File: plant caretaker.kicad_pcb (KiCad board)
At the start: 2 copper layers, 56 parts, among them J3 Water_Pump, J4 Kitronik, J5 694106402002, Q1 FDMS86255, U1 UDA1380HN_N2, U2 TMP175AIDR, U4 LM2596S-5, U5 PAM8403D, U6 ESP32_C3_ZERO

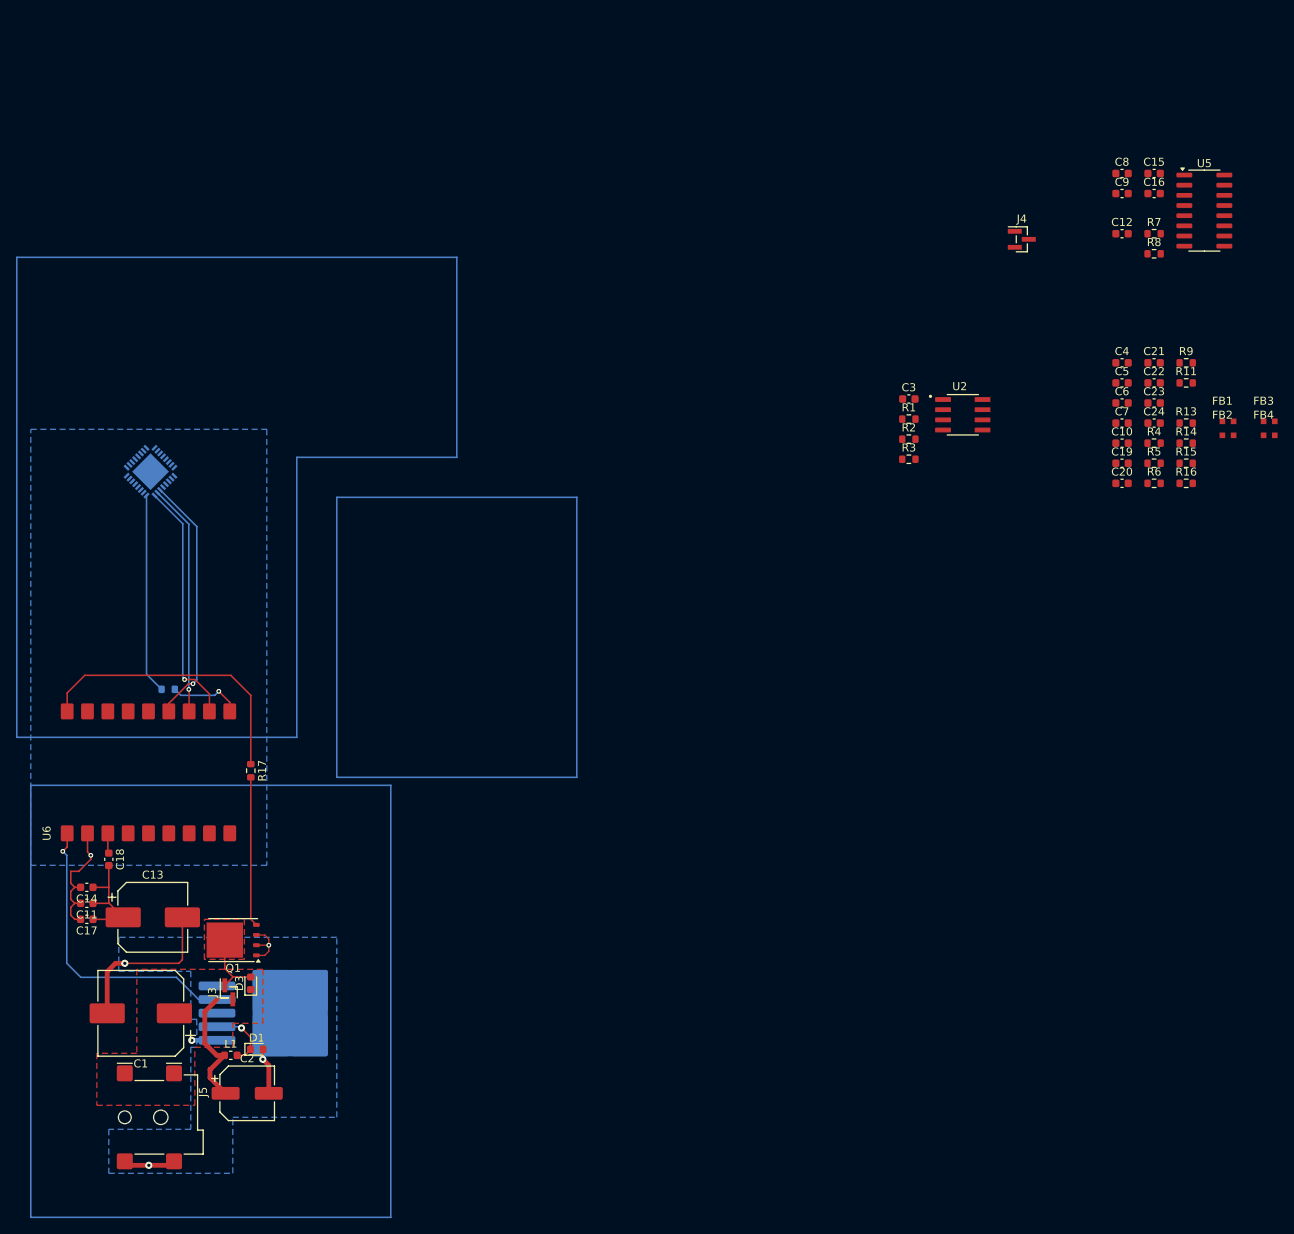
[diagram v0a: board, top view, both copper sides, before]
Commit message: Added more connections
Updated footprints for pin heads and speakers
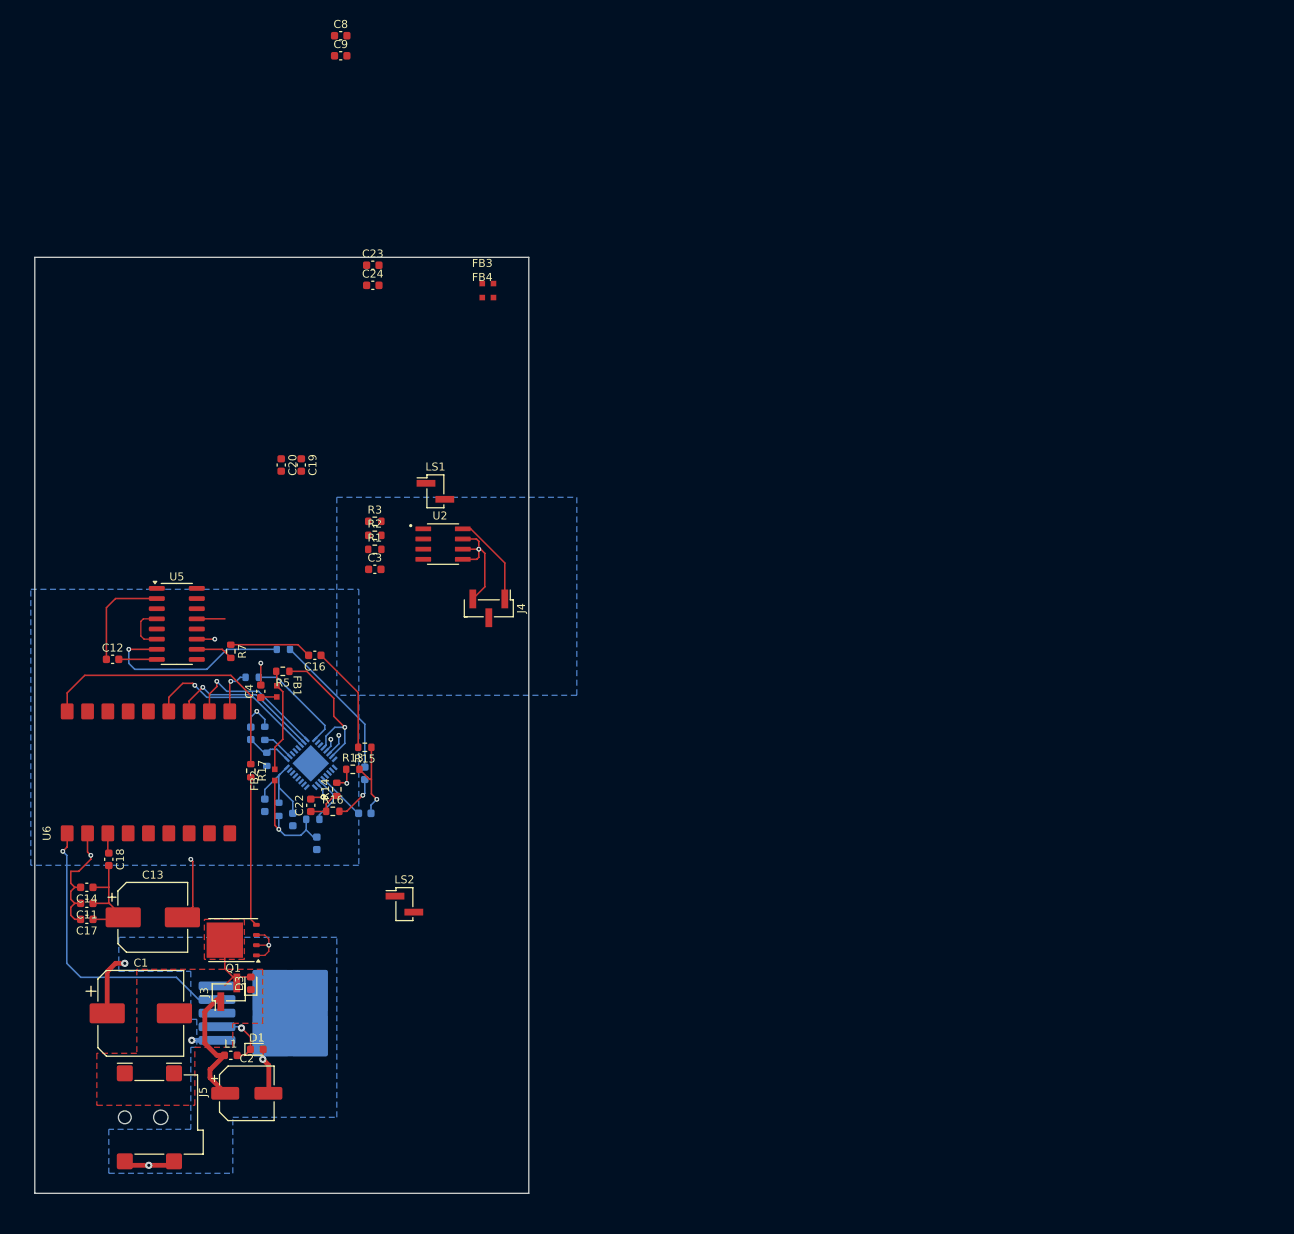
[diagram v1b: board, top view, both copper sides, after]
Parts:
- added LS1: Speaker, Connector_PinHeader_2.00mm:PinHeader_1x02_P2.00mm_Vertical_SMD_Pin1Left, F.Cu at (127.3, 54.2)
- added LS2: Speaker, Connector_PinHeader_2.00mm:PinHeader_1x02_P2.00mm_Vertical_SMD_Pin1Left, F.Cu at (123.5, 105.8)
- C10, C15, C21, C5, C6, C7, R11, R4, R6, R8, R9: moved to B.Cu
- J3: footprint Connector_PinHeader_1.00mm:PinHeader_1x02_P1.00mm_Vertical_SMD_Pin1Right -> Connector_PinHeader_2.00mm:PinHeader_1x02_P2.00mm_Vertical_SMD_Pin1Left
- J4: footprint Connector_PinHeader_1.00mm:PinHeader_1x03_P1.00mm_Vertical_SMD_Pin1Left -> Connector_PinHeader_2.00mm:PinHeader_1x03_P2.00mm_Vertical_SMD_Pin1Left
- moved U5 138.4 mm to (95.0, 70.8)
- moved C12 136.9 mm to (87.0, 75.2)
- moved R7 126.7 mm to (101.8, 74.2), turned to -90 degrees
- moved FB2 126.1 mm to (107.2, 90.4), turned to 90 degrees
- moved R9 124.1 mm to (106.0, 84.5), turned to 90 degrees
- moved C15 123.9 mm to (118.5, 89.5), turned to 90 degrees
- moved FB1 122.7 mm to (107.5, 78.5), turned to -90 degrees
- moved R11 122.0 mm to (112.0, 95.2), turned to 180 degrees
- moved C16 119.7 mm to (112.2, 74.8), turned to 180 degrees
- moved R8 119.5 mm to (108.3, 74.0), turned to 180 degrees
- moved R4 118.6 mm to (107.8, 94.0), turned to 90 degrees
- moved C6 118.4 mm to (106.0, 93.5), turned to 90 degrees
- moved C22 117.9 mm to (111.8, 93.5), turned to 90 degrees
- moved R6 116.2 mm to (106.2, 87.8), turned to 90 degrees
- moved C5 115.9 mm to (112.5, 98.2), turned to -90 degrees
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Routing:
- net +3V3: track 15.1 -> 49.2 mm
- net Net-(U5-INL): track 0.00 -> 25.1 mm, vias 0 -> 1
- net GND: track 55.3 -> 79.4 mm, vias 5 -> 9
- net /AudioCodec/A1: track 0.00 -> 19.9 mm, vias 0 -> 1
- net Net-(C15-Pad2): track 0.00 -> 18.6 mm
- net /AudioCodec/VDDA: track 0.00 -> 15.0 mm, vias 0 -> 1
- net /AudioAmplifier/R_IN: track 0.00 -> 13.4 mm
- net /AudioCodec/VADCP: track 0.00 -> 13.0 mm
- net /CODEC.DATAI: track 30.6 -> 18.4 mm
- net Net-(U1-SYSCLK): track 25.0 -> 13.2 mm
- net Net-(C21-Pad2): track 0.00 -> 10.8 mm, vias 0 -> 1
- net Net-(C16-Pad2): track 0.00 -> 10.3 mm
- net /CODEC.WSI: track 29.0 -> 19.2 mm
- net /CODEC.BCKI: track 31.4 -> 22.2 mm
- net /BuckConverter/12V: track 3.15 -> 11.0 mm, vias 1 -> 2
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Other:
- board outline added: 61.8 x 117 mm
